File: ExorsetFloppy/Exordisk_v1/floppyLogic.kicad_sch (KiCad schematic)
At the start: 92 parts, among them J10 Conn_01x01, J11 Conn_01x01, J12 Conn_01x01, J13 Conn_01x01, J14 Conn_01x01, J15 Conn_01x01, J16 Conn_01x01, J17 Conn_01x01, J18 Conn_01x01, J19 Conn_02x02_Odd_Even, J2 Floppy, J20 Conn_01x01, J21 Conn_01x01, J22 Conn_01x01, J23 Conn_01x01, J24 Conn_01x01, J25 Conn_01x01, J26 Conn_01x01, J27 Conn_01x01, J28 Conn_01x01, J29 Conn_01x01, J3 Conn_01x01, J30 Conn_01x01, J31 Conn_01x01, J32 Conn_01x01, J33 Conn_01x01, J34 Conn_01x01, J35 Conn_01x01, J36 Conn_01x01, J37 Conn_01x01, J38 Conn_01x01, J39 Conn_01x01, J40 Conn_01x01, J41 Conn_01x01, J7 Conn_01x17, J8 Conn_01x01, J9 Conn_01x01, Q1 BC337, U10 GAL16V8, U11 74HCT74, U12 74HCT74, U15 74HCT04, U16 74HCT74, U17 74HCT00, U18 74HCT74, U19 74LS112, U2 74HCT74, U20 68B21, U21 MC4024, U22 74LS157, U23 74LS123, U24 74HCT164, U25 74LS04, U27 MC4044, U28 74F163, U29 74F163, U34 6852_DIL24, U4 MC8506_new, U5 74F163, U6 74LS139, U7 74HCT240, U8 74HCT244, U9 74LS139

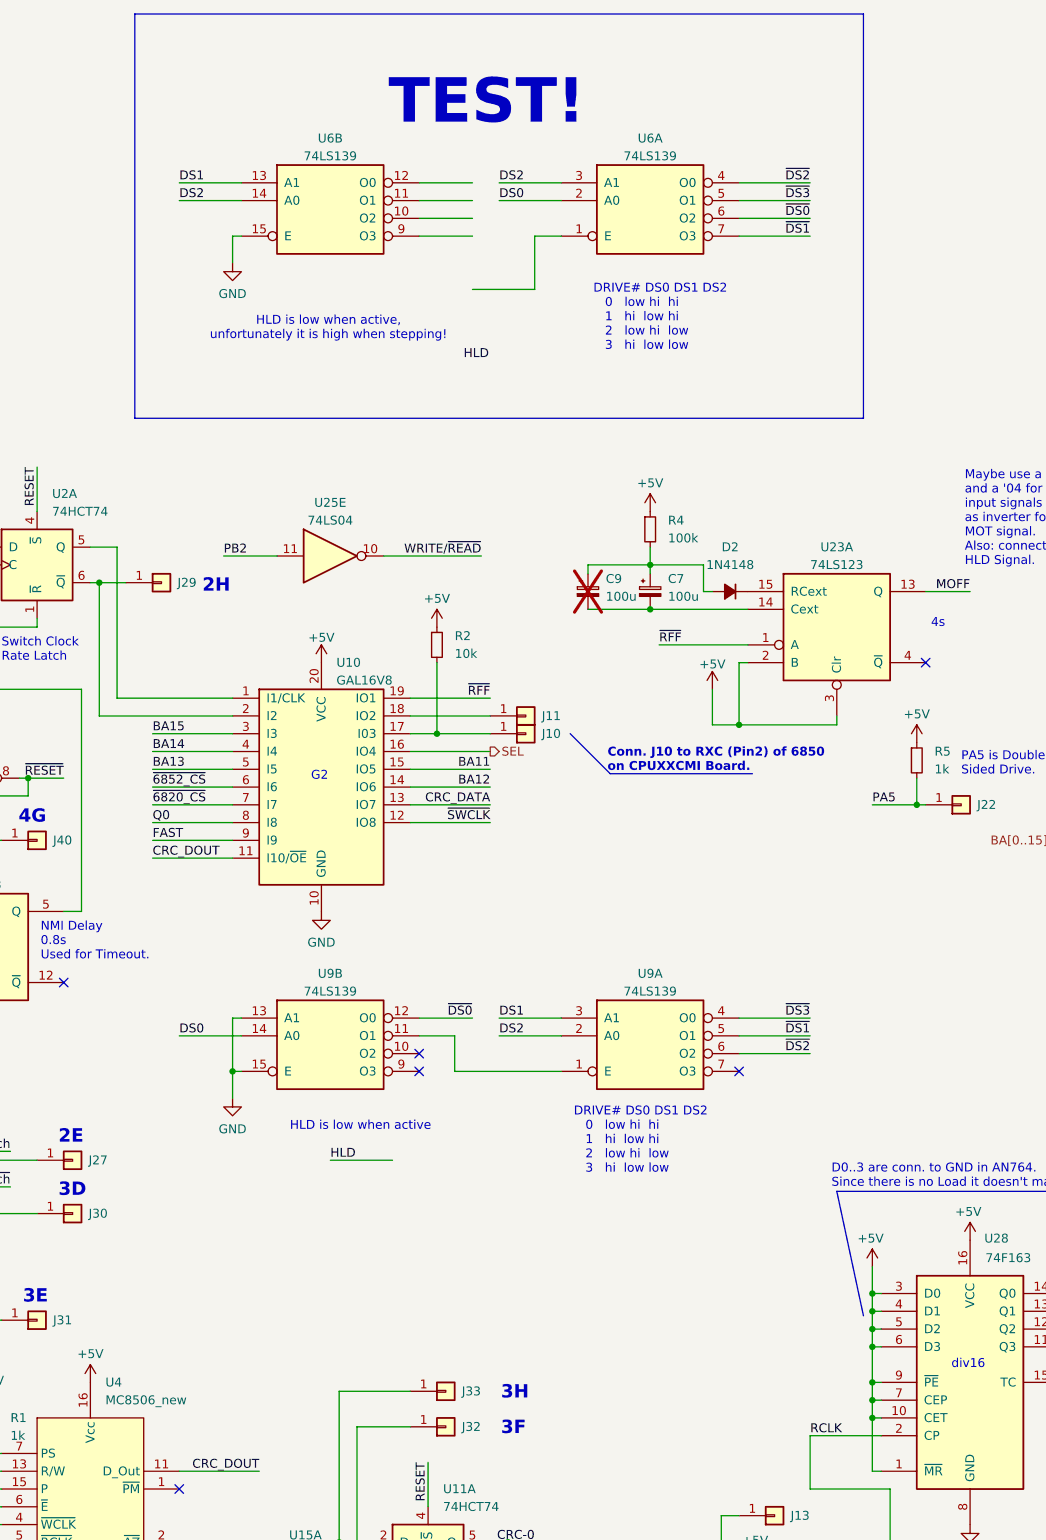
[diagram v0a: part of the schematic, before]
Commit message: Exordisk Board continued
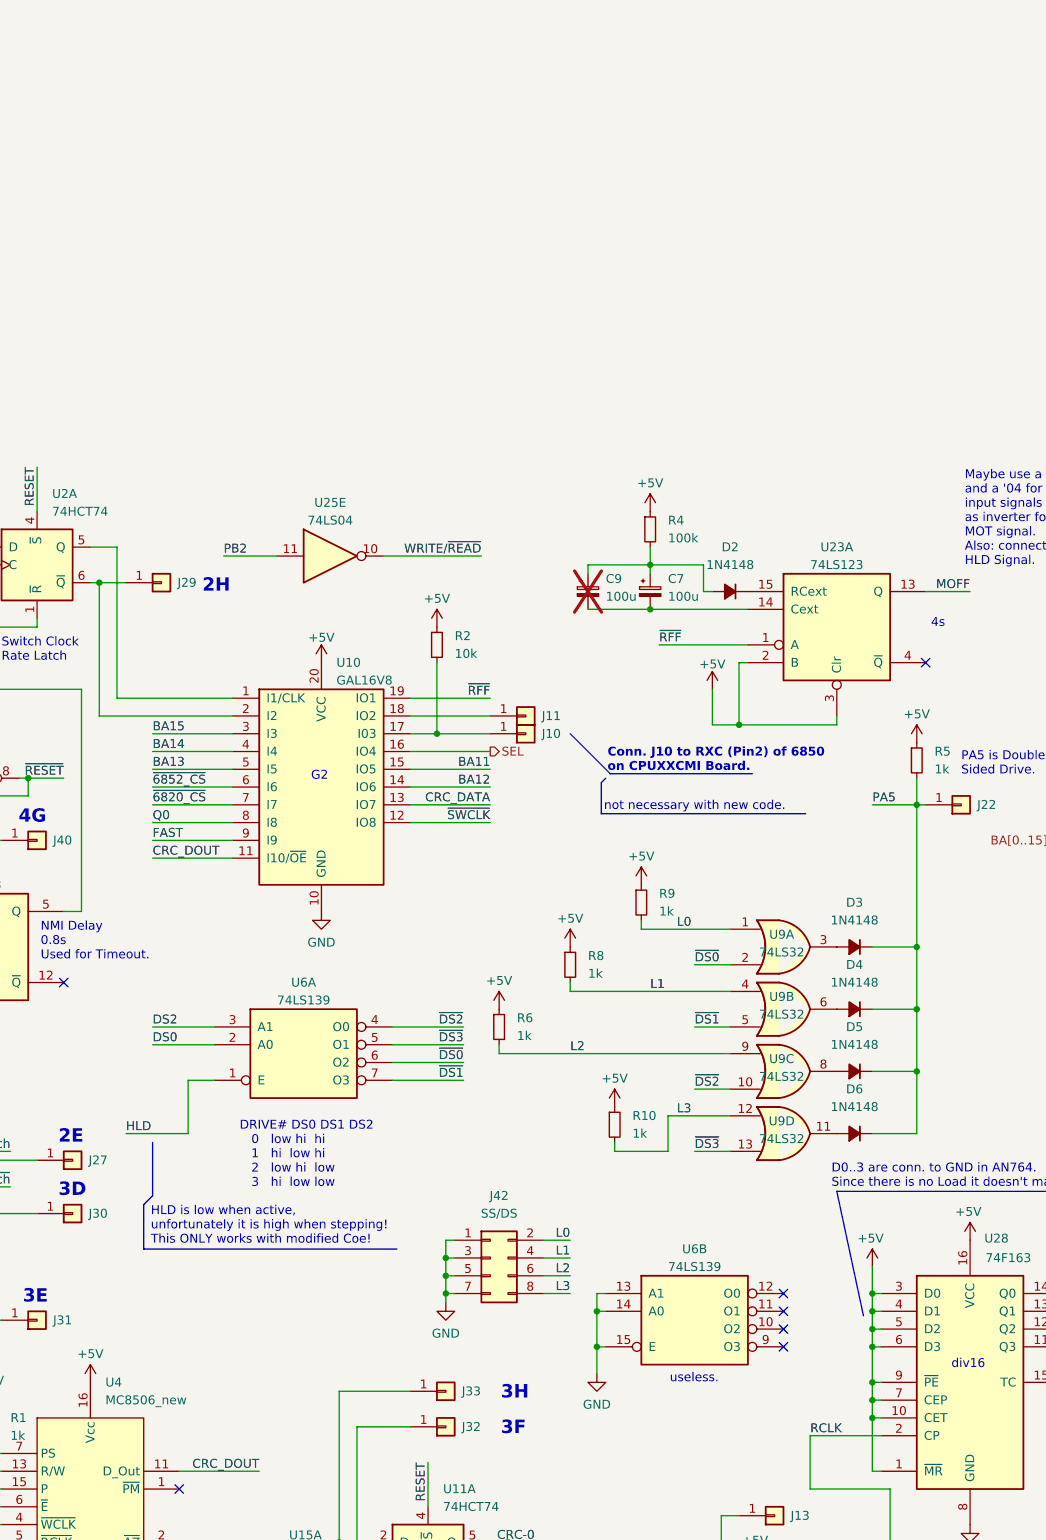
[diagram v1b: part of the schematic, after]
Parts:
- removed U9: 74LS139, Package_DIP:DIP-16_W7.62mm, symbol 74xx:74LS139
- added D3, D4, D5, D6: 1N4148, Diode_SMD:D_1206_3216Metric_Pad1.42x1.75mm_HandSolder, symbol Device:D_Small_Filled
- added J42: SS/DS, Connector_PinHeader_2.54mm:PinHeader_2x04_P2.54mm_Vertical, symbol Connector_Generic:Conn_02x04_Odd_Even
- added R10, R6, R8, R9: 1k, Resistor_SMD:R_1206_3216Metric_Pad1.30x1.75mm_HandSolder, symbol Device:R_Small
- added U9: 74LS32, Package_DIP:DIP-14_W7.62mm, symbol 74xx:74LS32
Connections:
- net +5V: now also R10.1, R6.1, R8.1, R9.1
- net DS1: no longer U6.13 (A1)
- net DS2: no longer U6.14 (A0)
- net GND: now also U6.13 (A1), U6.14 (A0), J42.1 (Pin_1), J42.3 (Pin_3), J42.5 (Pin_5), J42.7 (Pin_7)
- net HLD: now also U6.1 (E)
- net PA5: now also D3.1 (K), D4.1 (K), D5.1 (K), D6.1 (K)
- net ~{DS0}: now also U9.2
- net ~{DS1}: now also U9.5
- net ~{DS2}: now also U9.10
- net ~{DS3}: now also U9.13
- new net: D5.2 (A), U9.8
- new net: D4.2 (A), U9.6
- new net: D6.2 (A), U9.11
- new net: D3.2 (A), U9.3
- new net L0: J42.2 (Pin_2), R9.2, U9.1
- new net L1: J42.4 (Pin_4), R8.2, U9.4
- new net L2: J42.6 (Pin_6), R6.2, U9.9
- new net L3: J42.8 (Pin_8), R10.2, U9.12
- no-connect marks 42 -> 43
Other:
- note added: "HLD is low when active, unfortunately it is high when stepping! This ONLY works with modified Coe!"
- note added: "not necessary with new code."
- note added: "useless."
- note removed: "HLD is low when active"
- note removed: "HLD is low when active, unfortunately it is high when stepping!"
- note removed: "TEST!"
- moved on the sheet: U6A, U6B
